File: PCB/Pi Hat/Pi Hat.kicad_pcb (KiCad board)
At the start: 2 copper layers, 26.7 x 55.9 mm, 14 parts, among them IC1 MCP3008-I_SL, J1 Conn_01x04, J2 Conn_02x20_Odd_Even, J3 Conn_01x03, J4 Conn_01x02, U1 74LVC2T45DC

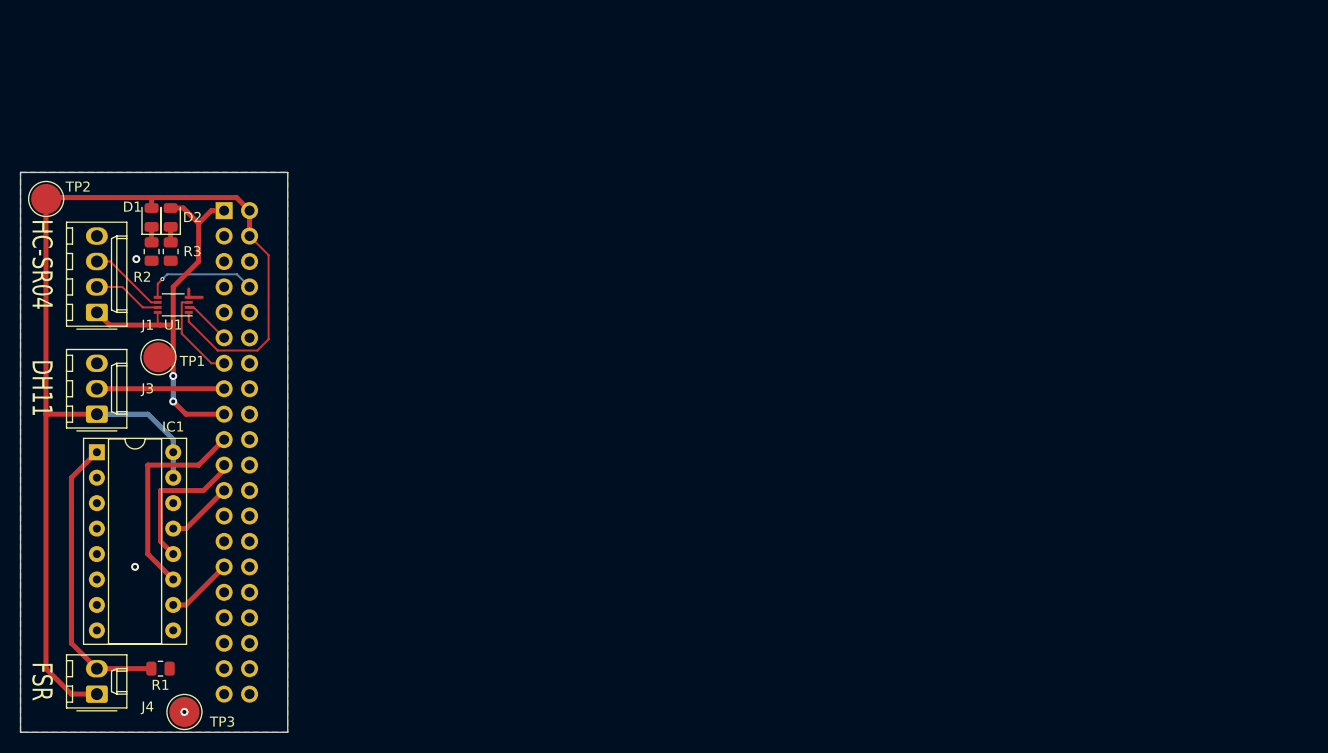
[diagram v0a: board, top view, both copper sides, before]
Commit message: complete PCB
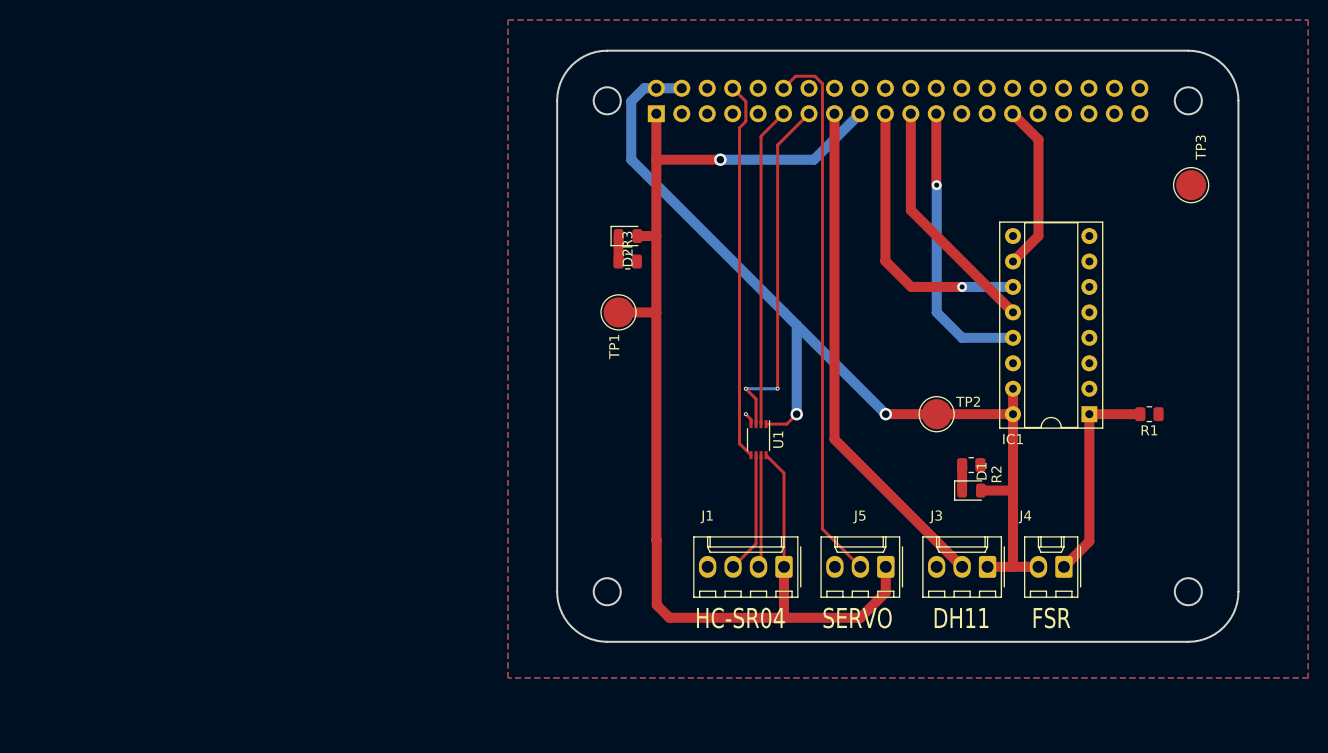
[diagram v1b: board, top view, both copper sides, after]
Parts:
- added J5: Conn_01x03, Connector_Molex:Molex_KK-254_AE-6410-03A_1x03_P2.54mm_Vertical, F.Cu at (177.8, 96.5)
- moved TP3 113.4 mm to (208.3, 58.4), turned to 90 degrees
- moved R1 101.9 mm to (204.1, 81.3)
- moved IC1 99.1 mm to (198.1, 81.3), turned to 180 degrees
- moved J4 97.4 mm to (195.6, 96.5), turned to 180 degrees
- moved TP2 91.4 mm to (182.9, 81.3)
- moved J3 90.2 mm to (188.0, 96.5), turned to 180 degrees
- moved D1 86.3 mm to (186.4, 88.9), turned to 0 degrees
- moved R2 84.5 mm to (186.3, 86.4), turned to 0 degrees
- moved J1 73.1 mm to (167.6, 96.5), turned to 180 degrees
- moved U1 59.9 mm to (165.1, 83.8), turned to -90 degrees
- moved TP1 46.1 mm to (151.1, 71.1), turned to -90 degrees
- moved D2 45.7 mm to (152.1, 63.5), turned to 0 degrees
- moved R3 45.6 mm to (152.0, 66.0), turned to 0 degrees
- moved J2 44.2 mm to (154.9, 51.3), turned to -90 degrees
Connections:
- J2 pad 12: unconnected-(J2-Pin_12-Pad12) -> /PWM_0
- J4 pad 1: +3.3V -> /ForceVoltage
- J4 pad 2: /ForceVoltage -> +3.3V
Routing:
- net +5V: track 41.9 -> 120.9 mm, vias 2 -> 1
- net /PWM_0: track 0.00 -> 54.5 mm
- net /Data_3.3VTTL: track 12.7 -> 50.5 mm
- net /Trigger_3.3VTTL: track 4.79 -> 31.9 mm
- net /Echo_3.3VTTL: track 9.25 -> 35.9 mm, vias 0 -> 2
- net /ConverterDir: track 11.4 -> 37.9 mm, vias 1 -> 0
- net /SCLK: track 6.65 -> 28.5 mm, vias 0 -> 1
- net +3.3V: track 116.7 -> 100.3 mm, vias 0 -> 2
- net /CS: track 6.65 -> 16.9 mm
- net /MISO: track 14.6 -> 24.1 mm
- net /ForceVoltage: track 29.1 -> 21.4 mm
- net /MOSI: track 21.2 -> 28.5 mm, vias 0 -> 1
- net /Trigger_5VTTL: track 6.91 -> 11.3 mm
- net /Echo_5VTTL: track 7.76 -> 12.1 mm
- net GND: track 2.20 -> 1.21 mm, vias 3 -> 1
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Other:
- board size 26.7 x 55.9 mm -> 68 x 59 mm
- board text added: "SERVO"
